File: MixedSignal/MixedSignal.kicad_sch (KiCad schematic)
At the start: 0 parts

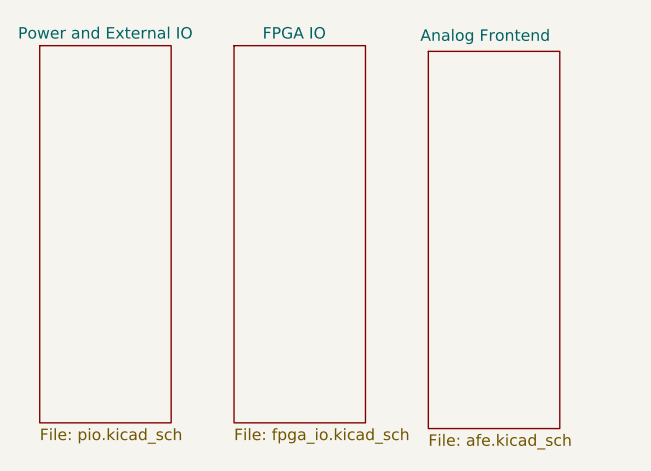
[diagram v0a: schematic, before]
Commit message: board rev. 1.1
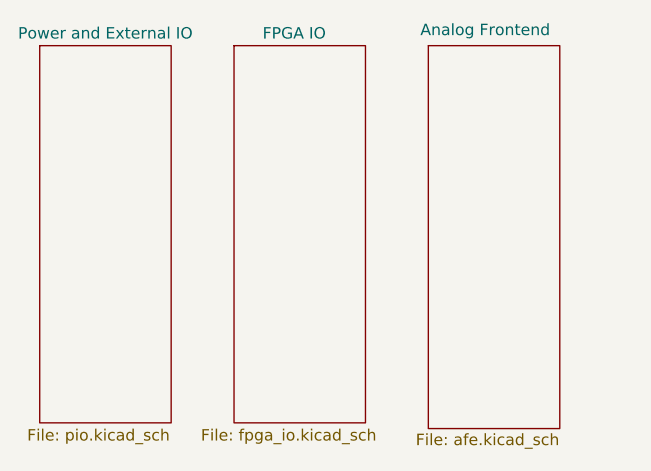
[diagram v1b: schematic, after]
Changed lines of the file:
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@@
 		)
 		(property "Sheetfile" "fpga_io.kicad_sch"
-			(at 201.295 69.7996 0)
+			(at 197.612 69.85 0)
 			(effects
 				(font
@@
 	)
 	(sheet
-		(at 222.885 27.94)
-		(size 14.605 41.91)
+		(at 222.885 27.305)
+		(size 14.605 42.545)
 		(stroke
 			(width 0.1524)
@@
 		)
 		(property "Sheetname" "Analog Frontend"
-			(at 221.996 26.924 0)
+			(at 221.996 26.289 0)
 			(effects
 				(font
@@
 		)
 		(property "Sheetfile" "afe.kicad_sch"
-			(at 222.885 70.4346 0)
+			(at 221.488 70.358 0)
 			(effects
 				(font
@@
 		)
 		(property "Sheetfile" "pio.kicad_sch"
-			(at 179.705 69.7996 0)
+			(at 178.308 69.85 0)
 			(effects
 				(font
